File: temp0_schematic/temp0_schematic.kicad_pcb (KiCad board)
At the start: 2 copper layers, 64 x 94 mm, 19 parts, among them J1 MODE_EXT, U1 Pro_Trinket_5V, U2 ESP-01, U3 oled_I2C_ssd1306, U4 hdc1080, U5 3.3V_REG, U6 ftdi_header

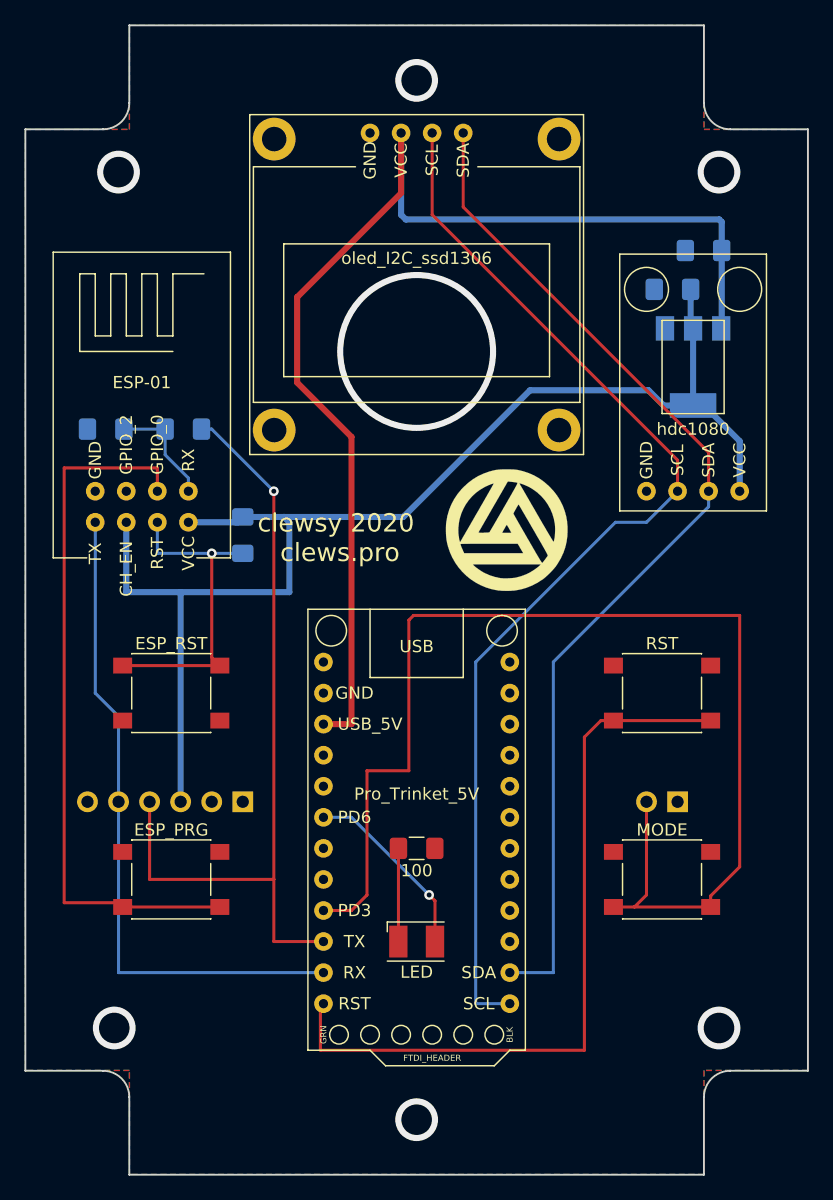
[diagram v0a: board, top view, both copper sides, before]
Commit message: Schematic and PCB revision 2.
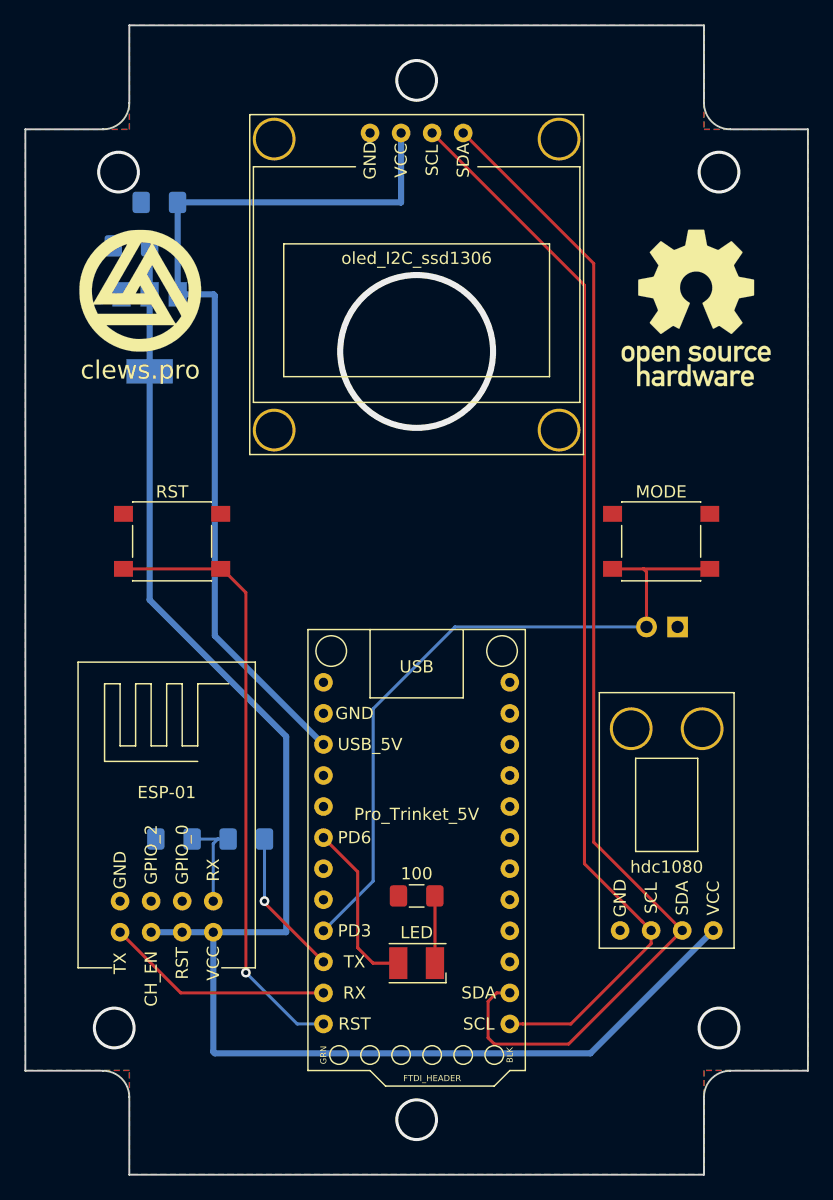
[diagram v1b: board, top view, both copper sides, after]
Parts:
- removed ESP_PRG, ESP_RST: SW_Push, Button_Switch_SMD:SW_Push_1P1T_NO_6x6mm_H9.5mm
- removed the G*** at (149.9, 92.1)
- removed R2: 10k, Resistor_SMD:R_1206_3216Metric_Pad1.42x1.75mm_HandSolder
- removed U6: ftdi_header, Connector_PinHeader_2.54mm:PinHeader_1x06_P2.54mm_Horizontal
- added G***: LOGO, temp0_parts:oshw_logo_10mm, F.Cu at (165.4, 73.9)
- added G***: LOGO, temp0_parts:oshw_logo_10mm, B.Cu at (160.3, 72.6)
- added G***: LOGO, temp0_parts:clewsy_logo_10mm, B.Cu at (142.7, 93.0)
- added G***: LOGO, temp0_parts:clewsy_logo_10mm, F.Cu at (119.9, 72.5)
- moved C1 44.7 mm to (121.4, 65.3)
- moved U5 44.5 mm to (120.7, 75.9)
- moved C2 44.4 mm to (119.2, 68.8)
- moved RST 41.9 mm to (122.5, 93.0)
- moved U4 35.9 mm to (162.9, 115.8)
- moved R3 34.0 mm to (122.6, 117.3)
- moved R4 33.9 mm to (128.6, 117.3)
- moved U2 33.6 mm to (122.0, 123.7)
- moved MODE 27.7 mm to (162.5, 93.0)
- moved J1 14.3 mm to (163.8, 100.0)
- moved R1 3.89 mm to (142.5, 122.0), turned to 180 degrees
- moved D1 1.77 mm to (142.5, 127.5), turned to 180 degrees
- moved U1 1.66 mm to (142.5, 118.5)
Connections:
- U2 pad 6: Net-(ESP_RST1-Pad1) -> 3.3V
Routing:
- net Net-(U2-Pad5): track 58.0 -> 0.00 mm
- net U1_TX: track 65.4 -> 12.0 mm
- net Net-(J1-Pad2): track 99.0 -> 57.8 mm
- net U1_RX: track 54.4 -> 18.7 mm
- net Net-(ESP_RST1-Pad1): track 26.9 -> 0.00 mm, vias 1 -> 0
- net 5V: track 97.9 -> 75.0 mm
- net 3.3V: track 107.5 -> 126.7 mm
- net Net-(RST1-Pad2): track 62.1 -> 50.0 mm, vias 0 -> 1
- net SDA: track 85.8 -> 97.6 mm
- net SCL: track 90.6 -> 88.0 mm
- net Net-(D1-Pad1): track 7.63 -> 5.51 mm
- net Net-(D1-Pad2): track 15.3 -> 14.0 mm, vias 1 -> 0
- net Net-(R3-Pad1): track 9.24 -> 8.18 mm
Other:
- board text added: "2"
- board text added: "clews.pro"
- board text added: "temp0 PCB layout"
- board text removed: "BLK"
- board text removed: "GRN"
- board text removed: "clewsy 2020 clews.pro"
